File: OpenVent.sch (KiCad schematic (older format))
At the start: 0 parts

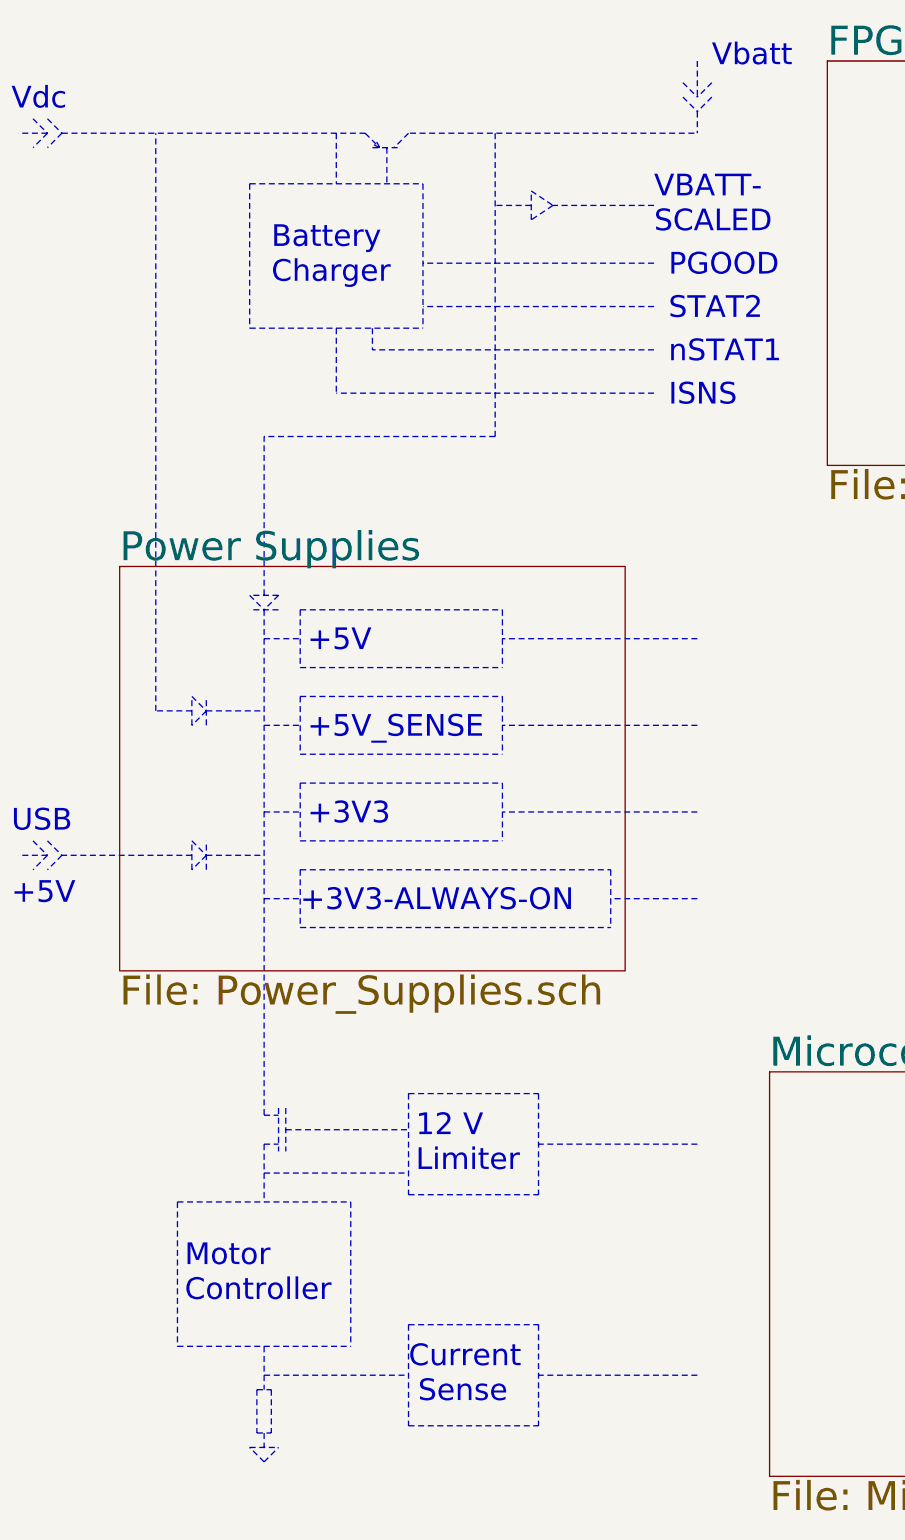
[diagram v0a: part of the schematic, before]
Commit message: Successful merge of Shrookie's changes to main
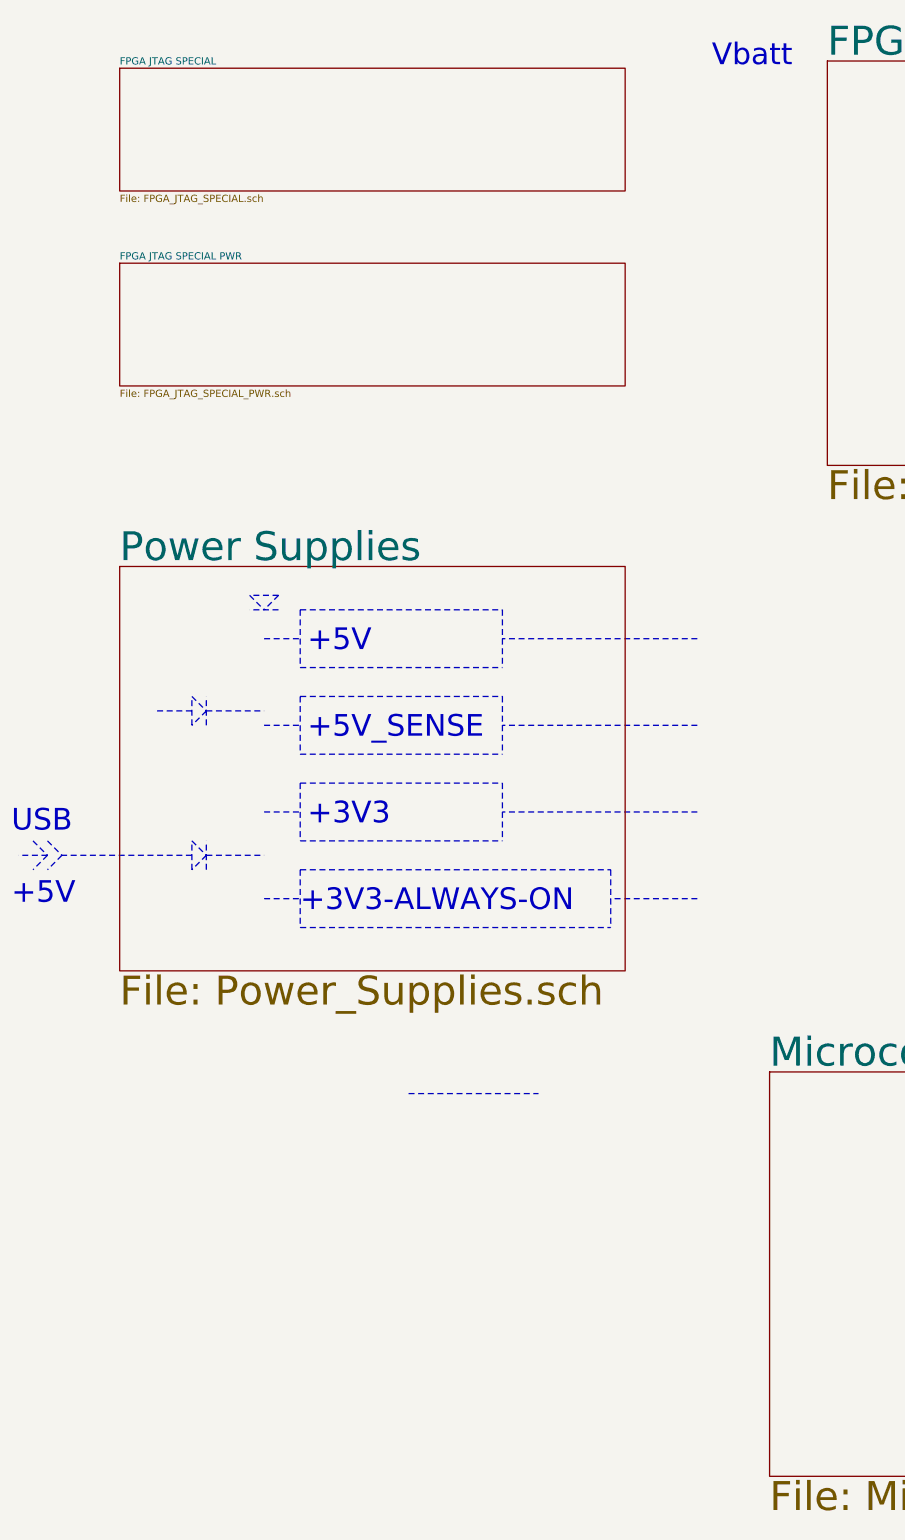
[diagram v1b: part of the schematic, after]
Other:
- note removed: "12 V\nLimiter"
- note removed: "Battery\nCharger"
- note removed: "Current\n Sense"
- note removed: "ISNS"
- note removed: "Motor\nController"
- note removed: "PGOOD"
- note removed: "STAT2"
- note removed: "VBATT-\nSCALED"
- note removed: "Vdc"
- note removed: "nSTAT1"
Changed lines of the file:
@@
 $Descr A3 16535 11693
 encoding utf-8
-Sheet 1 6
+Sheet 1 8
 Title "OpenVent Control Board"
 Date "2020-10-20"
@@
 MCU
 Wire Notes Line style solid
-	2500 8300 2600 8300
-Wire Notes Line style solid
-	2500 8500 2600 8500
-Wire Notes Line style solid
-	2600 8250 2600 8550
-Wire Notes Line style solid
-	2650 8250 2650 8550
-Wire Notes Line style solid
-	1900 8900 1900 9900
-Wire Notes Line style solid
-	3100 8900 3100 9900
-Wire Notes Line style solid
-	1900 9900 3100 9900
-Wire Notes Line style solid
-	1900 8900 3100 8900
-Wire Notes Line style solid
-	2500 8500 2500 8900
-Wire Notes Line style solid
-	3500 8150 3500 8850
-Wire Notes Line style solid
-	4400 8150 4400 8850
-Wire Notes Line style solid
-	3500 8850 4400 8850
-Wire Notes Line style solid
 	3500 8150 4400 8150
-Wire Notes Line style solid
-	2650 8400 3500 8400
-Text Notes 3550 8700 0    150  ~ 0
- 12 V\nLimiter
-Wire Notes Line style solid
-	2500 8700 3500 8700
-Wire Notes Line style solid
-	3500 9750 3500 10450
-Wire Notes Line style solid
-	4400 9750 4400 10450
-Wire Notes Line style solid
-	3500 10450 4400 10450
-Wire Notes Line style solid
-	3500 9750 4400 9750
-Text Notes 3500 10300 0    150  ~ 0
-Current\n Sense
-Wire Notes Line style solid
-	2500 9900 2500 10200
-Wire Notes Line style solid
-	2500 10100 3500 10100
-Text Notes 1950 9600 0    150  ~ 0
-  Motor\nController
-Wire Notes Line style solid
-	2450 10200 2450 10500
-Wire Notes Line style solid
-	2550 10200 2550 10500
-Wire Notes Line style solid
-	2450 10500 2550 10500
-Wire Notes Line style solid
-	2450 10200 2550 10200
-Wire Notes Line style solid
-	2400 10600 2600 10600
-Wire Notes Line style solid
-	2500 10500 2500 10600
-Wire Notes Line style solid
-	2500 10700 2600 10600
-Wire Notes Line style solid
-	2500 10700 2400 10600
-Wire Notes Line style solid
-	2400 1850 2400 2850
-Wire Notes Line style solid
-	3600 1850 3600 2850
-Wire Notes Line style solid
-	2400 1850 3600 1850
-Wire Notes Line style solid
-	3000 1500 3000 1850
-Text Notes 2550 2550 0    150  ~ 0
-Battery\nCharger
-Wire Notes Line style solid
-	1750 5500 1750 1500
-Wire Notes Line style solid
-	1100 1500 1000 1600
-Wire Notes Line style solid
-	1000 1400 1100 1500
-Wire Notes Line style solid
-	1000 1500 900  1600
-Wire Notes Line style solid
-	900  1400 1000 1500
-Wire Notes Line style solid
-	1000 1500 800  1500
-Text Notes 750  1350 0    150  ~ 0
-Vdc
 Text Notes 750  6350 0    150  ~ 0
 USB
@@
 Wire Notes Line style solid
 	2600 4700 2400 4700
-Wire Notes Line style solid
-	2500 4700 2500 3600
-Wire Notes Line style solid
-	2500 4800 2500 8300
-Wire Notes Line style solid
-	4100 3600 2500 3600
-Wire Notes Line style solid
-	5500 1350 5500 1500
-Wire Notes Line style solid
-	5600 1250 5500 1350
-Wire Notes Line style solid
-	5400 1250 5500 1350
-Wire Notes Line style solid
-	5600 1150 5500 1250
-Wire Notes Line style solid
-	5400 1150 5500 1250
-Wire Notes Line style solid
-	5500 1000 5500 1250
 Text Notes 5600 1050 0    150  ~ 0
 Vbatt
-Wire Notes Line style solid
-	4500 2000 4350 2100
-Wire Notes Line style solid
-	4350 1900 4500 2000
-Wire Notes Line style solid
-	4350 2100 4350 1900
-Wire Notes Line style solid
-	4350 2000 4100 2000
-Wire Notes Line style solid
-	5200 2000 4500 2000
-Text Notes 5200 2200 0    150  ~ 0
-VBATT-\nSCALED
-Text Notes 5300 2500 0    150  ~ 0
-PGOOD
-Wire Notes Line style solid
-	5200 2400 3600 2400
-Text Notes 5300 2800 0    150  ~ 0
-STAT2
-Text Notes 5300 3100 0    150  ~ 0
-nSTAT1
-Wire Notes Line style solid
-	4100 1500 4100 3600
-Text Notes 5300 3400 0    150  ~ 0
-ISNS
-Wire Notes Line style solid
-	2400 2850 3600 2850
-Wire Notes Line style solid
-	5200 2700 3600 2700
-Wire Notes Line style solid
-	5200 3000 3250 3000
-Wire Notes Line style solid
-	5200 3300 3000 3300
-Wire Notes Line style solid
-	3250 2850 3250 3000
 Wire Notes Line style solid
 	2750 4800 2750 5200
@@
 	5500 6800 4900 6800
 Wire Notes Line style solid
-	5500 8500 4400 8500
-Wire Notes Line style solid
-	5500 10100 4400 10100
-Wire Notes Line style solid
 	2100 6500 2500 6500
 Wire Notes Line style solid
@@
 $EndSheet
 Wire Notes Line style solid
-	3200 1500 3300 1600
-Wire Notes Line style solid
-	3500 1500 3400 1600
-Wire Notes Line style solid
-	3250 1600 3450 1600
-Wire Notes Line style solid
-	3350 1600 3350 1850
-Wire Notes Line style solid
-	3280 1560 3300 1600
-Wire Notes Line style solid
-	3260 1580 3300 1600
-Wire Notes Line style solid
-	3510 1500 5500 1500
-Wire Notes Line style solid
-	1100 1500 3200 1500
-Wire Notes Line style solid
 	10000 10750 10000 11000
 Text Notes 10050 11100 0    150  ~ 0
@@
 Wire Notes Line style solid
 	10900 9750 10900 10650
-Wire Notes Line style solid
-	3000 2850 3000 3300
 Wire Notes Line style solid
 	15600 1400 15500 1500
@@
 Text Notes 11350 7850 0    150  ~ 0
 JMPR
+$Sheet
+S 1500 1050 3500 850
+U 5FBE832C
+F0 "FPGA JTAG SPECIAL" 50
+F1 "FPGA_JTAG_SPECIAL.sch" 50
+$EndSheet
+$Sheet
+S 1500 2400 3500 850
+U 5FBE8499
+F0 "FPGA JTAG SPECIAL PWR" 50
+F1 "FPGA_JTAG_SPECIAL_PWR.sch" 50
+$EndSheet
 $EndSCHEMATC

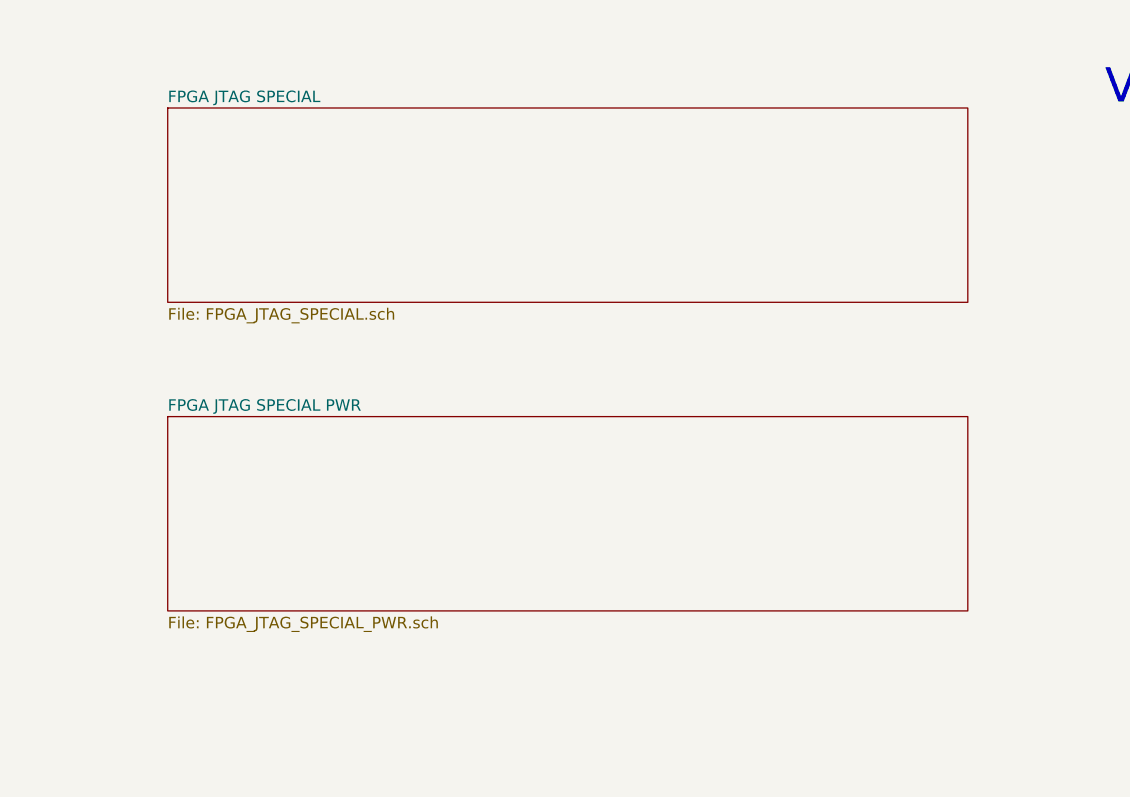
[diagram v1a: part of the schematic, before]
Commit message: Stuff
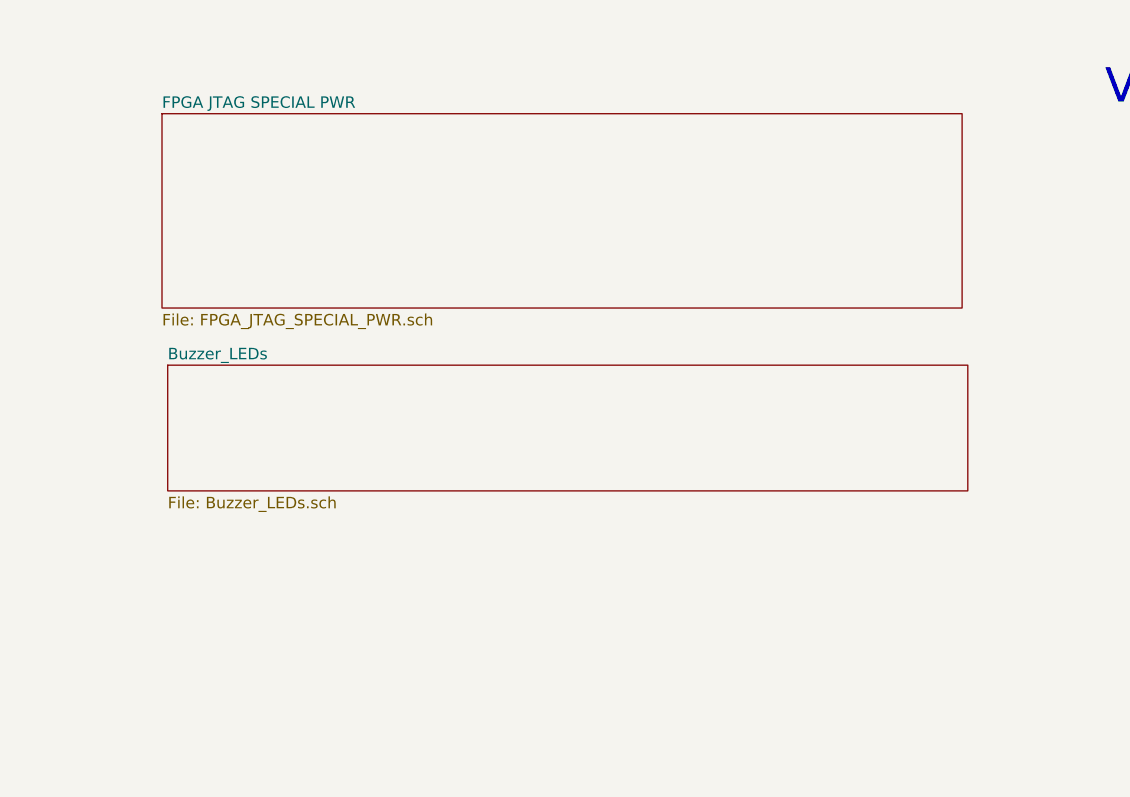
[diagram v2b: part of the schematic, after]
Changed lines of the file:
@@
 JMPR
 $Sheet
-S 1500 1050 3500 850
-U 5FBE832C
-F0 "FPGA JTAG SPECIAL" 50
-F1 "FPGA_JTAG_SPECIAL.sch" 50
-$EndSheet
-$Sheet
-S 1500 2400 3500 850
+S 1475 1075 3500 850
 U 5FBE8499
 F0 "FPGA JTAG SPECIAL PWR" 50
 F1 "FPGA_JTAG_SPECIAL_PWR.sch" 50
 $EndSheet
+$Sheet
+S 1500 2175 3500 550
+U 5FCA4074
+F0 "Buzzer_LEDs" 50
+F1 "Buzzer_LEDs.sch" 50
+$EndSheet
 $EndSCHEMATC
